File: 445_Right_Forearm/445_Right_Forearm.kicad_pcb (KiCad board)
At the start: 2 copper layers, 24.9 x 18 mm, 2 parts, among them J1 69167-107HLF, U1 LSM6DSMTR

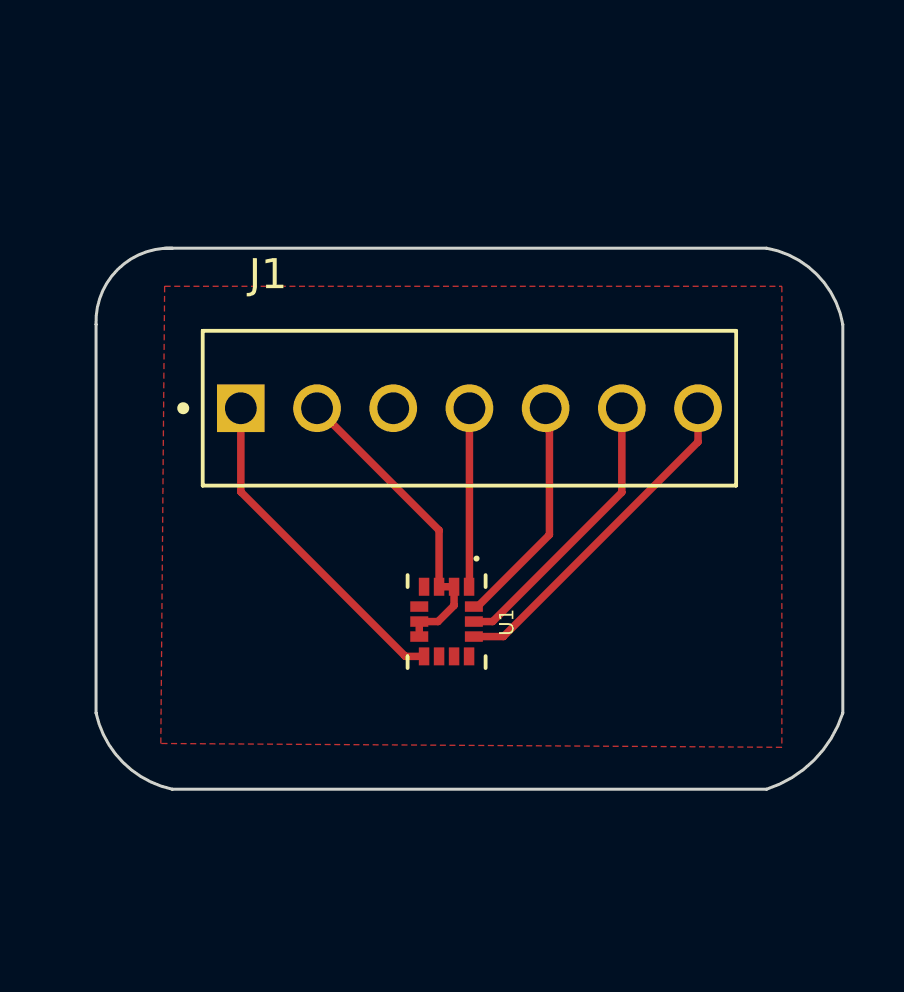
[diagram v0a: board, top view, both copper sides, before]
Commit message: Layout First Draft
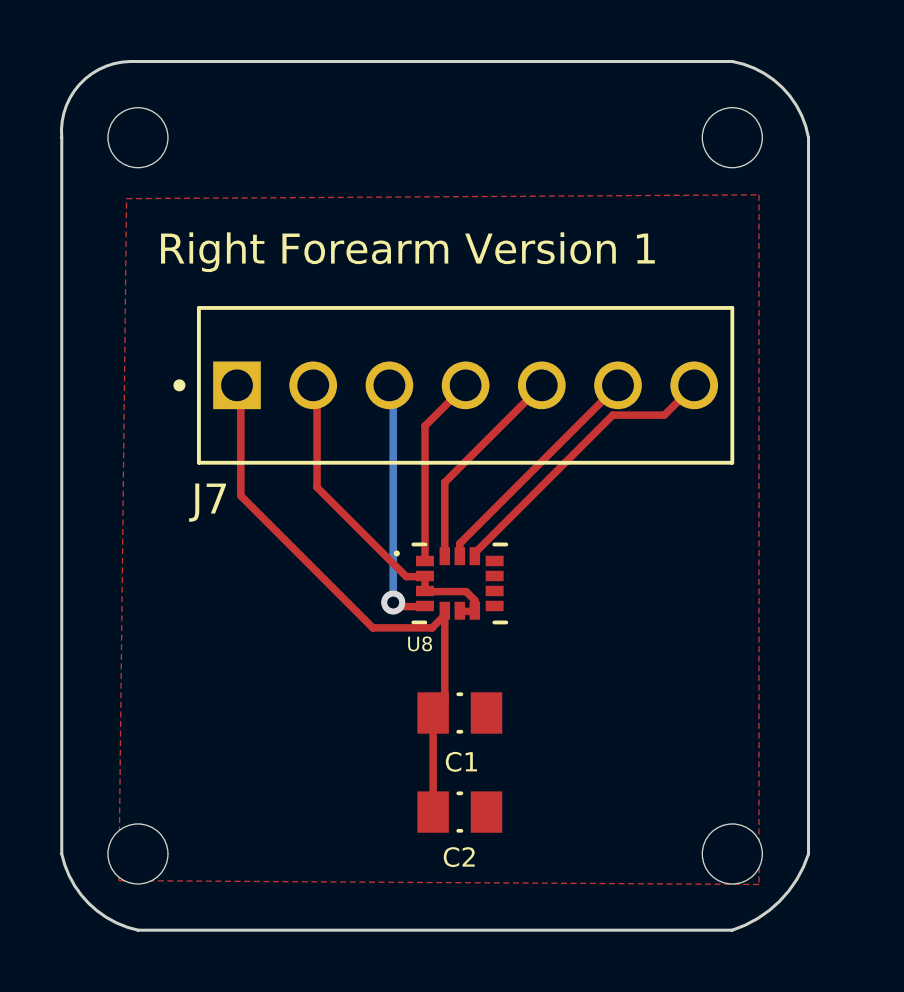
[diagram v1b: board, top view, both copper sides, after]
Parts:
- removed J1: 69167-107HLF, 69167-107HLF:AMPHENOL_69167-107HLF
- removed U1: LSM6DSMTR, LSM6DSMTR (1):PQFN50P300X250X86-14N
- added C1: 100nF, CL21F104ZAANNNC:CAPC2012X135N, F.Cu at (145.6, 92.8)
- added C2: 100nF, CL21F104ZAANNNC:CAPC2012X135N, F.Cu at (145.6, 96.1)
- added H1: MountingHole, MountingHole:MountingHole_2mm, F.Cu at (134.9, 73.7)
- added H2: MountingHole, MountingHole:MountingHole_2mm, F.Cu at (154.7, 73.7)
- added H3: MountingHole, MountingHole:MountingHole_2mm, F.Cu at (134.9, 97.5)
- added H4: MountingHole, MountingHole:MountingHole_2mm, F.Cu at (154.7, 97.5)
- added J7: 69167-107HLF, 69167-107HLF:AMPHENOL_69167-107HLF, F.Cu at (145.8, 81.9)
- added U8: LSM6DSMTR, LSM6DSMTR (1):PQFN50P300X250X86-14N, F.Cu at (145.6, 88.5)
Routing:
- net /CS2: track 11.3 -> 0.00 mm
- net /SENSOR_3: track 0.00 -> 9.93 mm
- net /CLK: track 9.52 -> 0.00 mm
- net /INT1_3: track 0.00 -> 8.48 mm, vias 0 -> 1
- net +3.3V: track 11.2 -> 19.4 mm
- net /CLK3: track 0.00 -> 8.08 mm
- net /MOSI: track 7.78 -> 0.00 mm
- net /MOSI_3: track 0.00 -> 7.23 mm
- net /MISO_3: track 0.00 -> 6.62 mm
- net /MISO: track 5.96 -> 0.00 mm
- net GND: track 10.6 -> 11.5 mm
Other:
- board size 24.9 x 18 mm -> 24.9 x 29 mm
- board text added: "Right Forearm Version 1"
